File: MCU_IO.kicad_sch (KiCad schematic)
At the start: 32 parts, among them J8 Conn_01x02, Q1 IRLML2803, SW1 SW_Omron_B3FS, SW2 SW_Omron_B3FS, U1 MR25H40MDF, U2 RP2040, U3 MAX706RESA+, Y1 12MHz

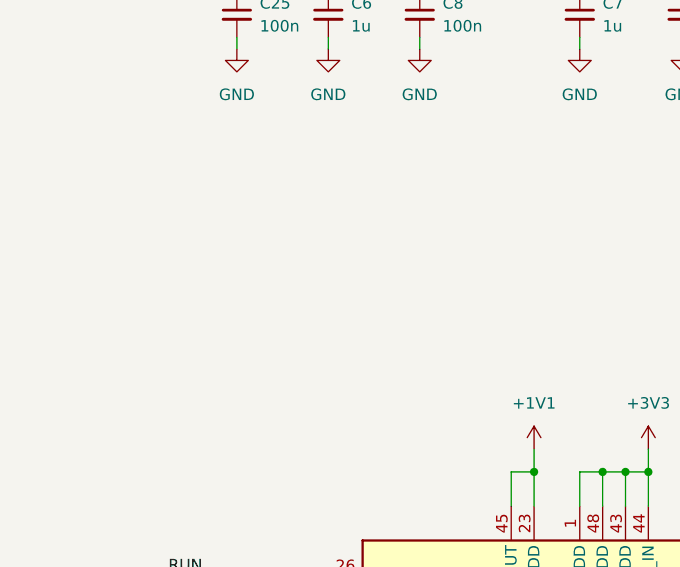
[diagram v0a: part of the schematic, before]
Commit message: Fixed schematic bugs and corresponding layout modifications
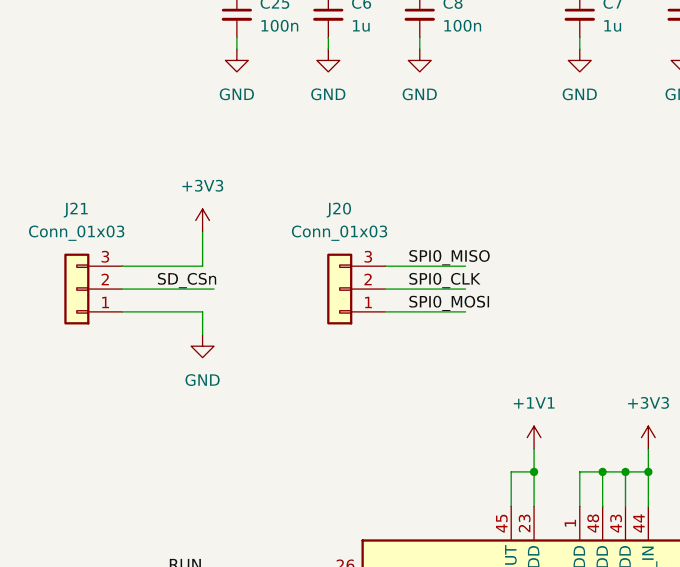
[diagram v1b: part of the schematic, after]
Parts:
- added J20: Conn_01x03, Connector_PinSocket_2.54mm:PinSocket_1x03_P2.54mm_Vertical, symbol Connector_Generic:Conn_01x03
- added J21: Conn_01x03, Connector_PinHeader_2.54mm:PinHeader_1x03_P2.54mm_Vertical, symbol Connector_Generic:Conn_01x03
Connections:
- net +3V3: now also J21.3 (Pin_3)
- net GND: now also J21.1 (Pin_1)
- net SD_CSn: now also J21.2 (Pin_2)
- net SPI0_CLK: now also J20.2 (Pin_2)
- net SPI0_MISO: now also J20.3 (Pin_3)
- net SPI0_MOSI: now also J20.1 (Pin_1)

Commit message: Updated connector locations and types
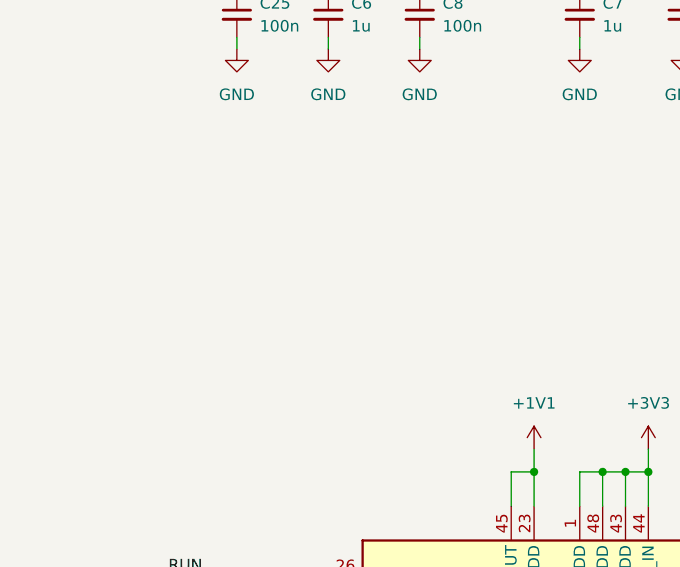
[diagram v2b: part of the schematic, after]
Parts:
- removed J20: Conn_01x03, Connector_PinSocket_2.54mm:PinSocket_1x03_P2.54mm_Vertical, symbol Connector_Generic:Conn_01x03
- removed J21: Conn_01x03, Connector_PinHeader_2.54mm:PinHeader_1x03_P2.54mm_Vertical, symbol Connector_Generic:Conn_01x03
